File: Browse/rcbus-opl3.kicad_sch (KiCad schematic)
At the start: 37 parts, among them CON1 SJ1-3523N, P1 RC2014 BUS, U1 74HCT688, U2 YMF262, U3 YAC512, U4 TL074, Y1 SG-8002CA

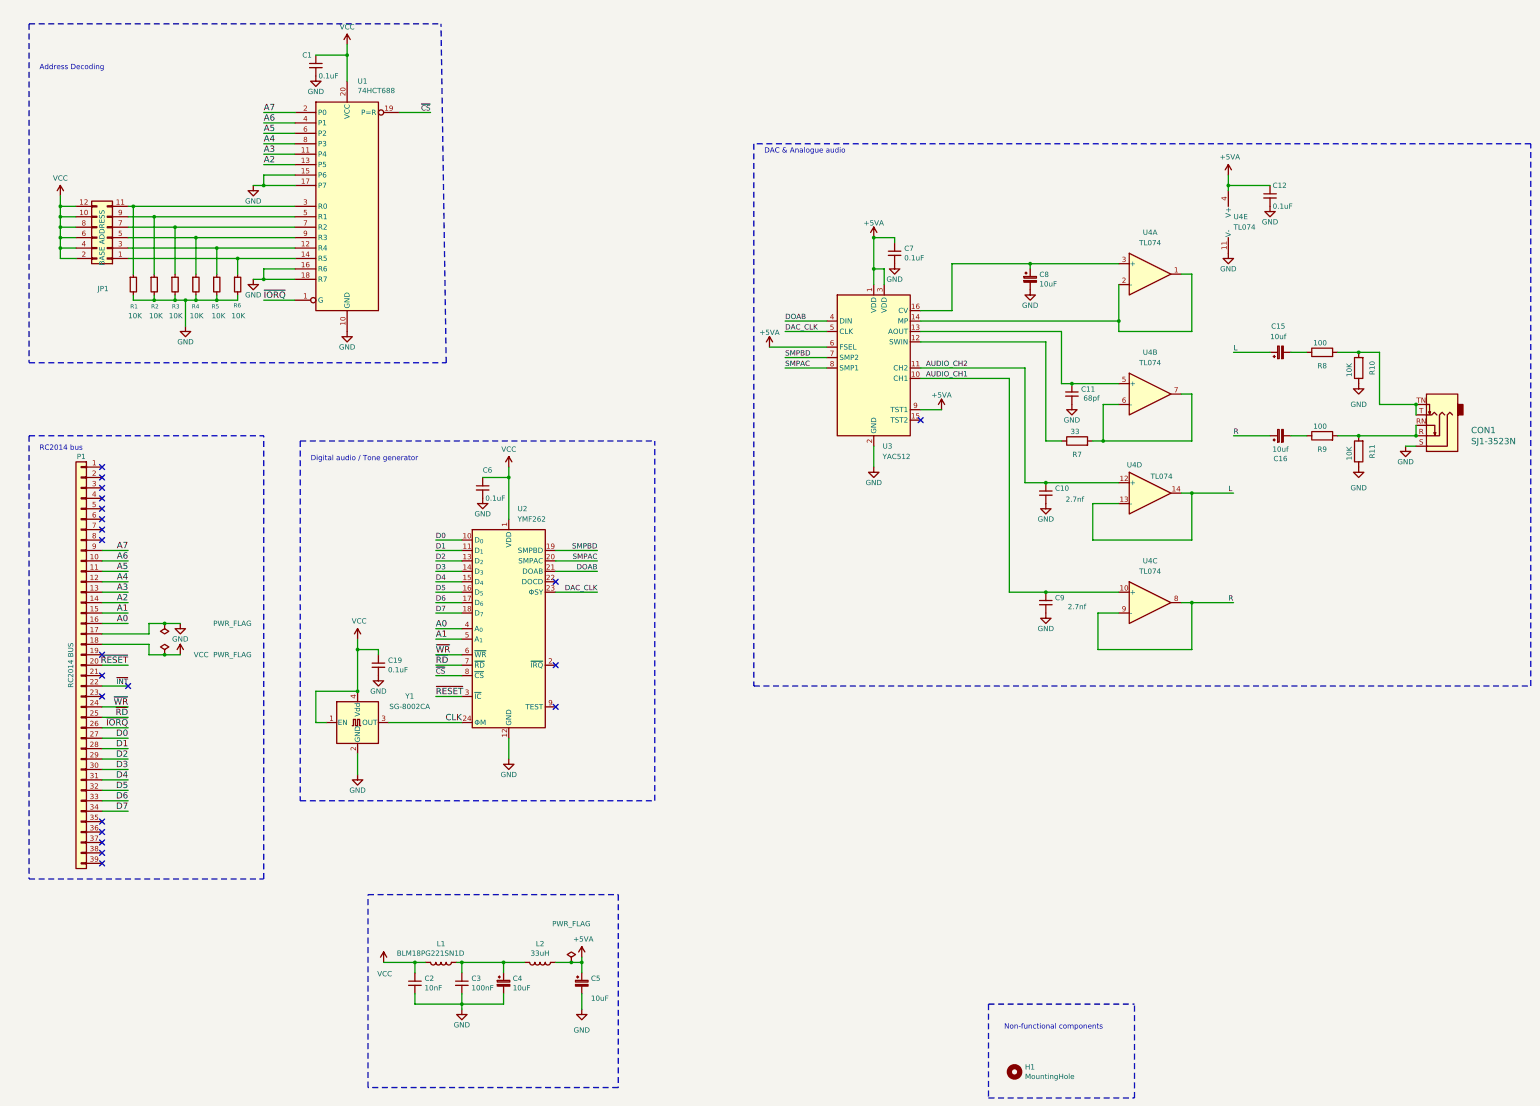
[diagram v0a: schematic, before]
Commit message: Deploying to main from @ electrified/rcbus-opl3@ca335f471b0cc053c0f7ada637c7f1deac17d0b8 🚀
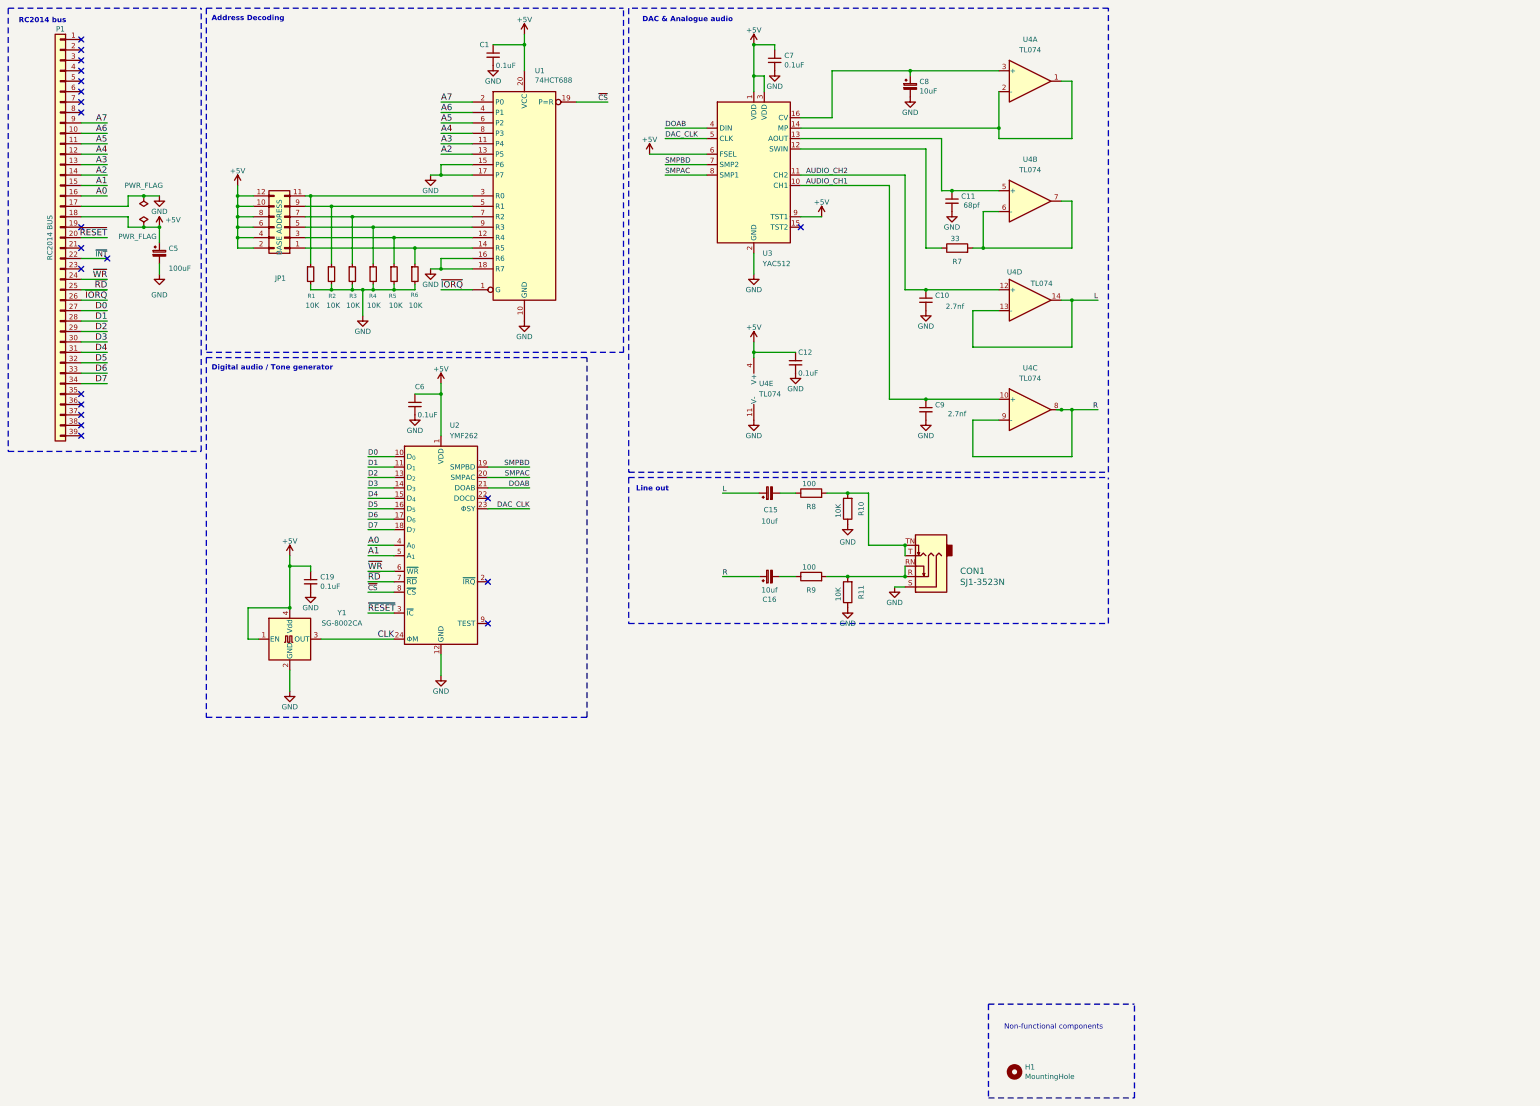
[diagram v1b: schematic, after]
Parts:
- removed C2: 10nF, Capacitor_SMD:C_0603_1608Metric, symbol Device:C_Small
- removed C3: 100nF, Capacitor_SMD:C_0603_1608Metric, symbol Device:C_Small
- removed C4: 10uF, Capacitor_SMD:C_1206_3216Metric, symbol Device:C_Polarized_Small
- removed L1: BLM18PG221SN1D, Inductor_SMD:L_0603_1608Metric, symbol Device:L
- removed L2: 33uH, Inductor_SMD:L_0603_1608Metric, symbol Device:L
- C15, C16: footprint Capacitor_SMD:CP_Elec_5x5.9 -> Capacitor_SMD:CP_Elec_6.3x5.8
- C5: value 10uF -> 100uF; footprint Capacitor_SMD:C_1206_3216Metric -> Capacitor_SMD:CP_Elec_6.3x7.7
- C8: footprint Capacitor_SMD:C_0603_1608Metric -> Capacitor_SMD:CP_Elec_6.3x5.8
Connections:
- net VCC is gone; now on net +5V: C1.1, C19.1, C6.1, JP1.10 (Pin_10), JP1.12 (Pin_12), JP1.2 (Pin_2), JP1.4 (Pin_4), JP1.6 (Pin_6), JP1.8 (Pin_8), P1.18 (Pin_18), U1.20 (VCC), U2.1 (VDD), Y1.1 (EN), Y1.4 (Vdd)
- net +5VA renamed +5V
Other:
- note added: "Line out"
- moved on the sheet: C1, C10, C11, C12, C15, C16, C19, C5, C6, C7, C8, C9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
